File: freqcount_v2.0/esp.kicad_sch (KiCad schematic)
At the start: 1 part, among them J3 Conn_02x10_Odd_Even

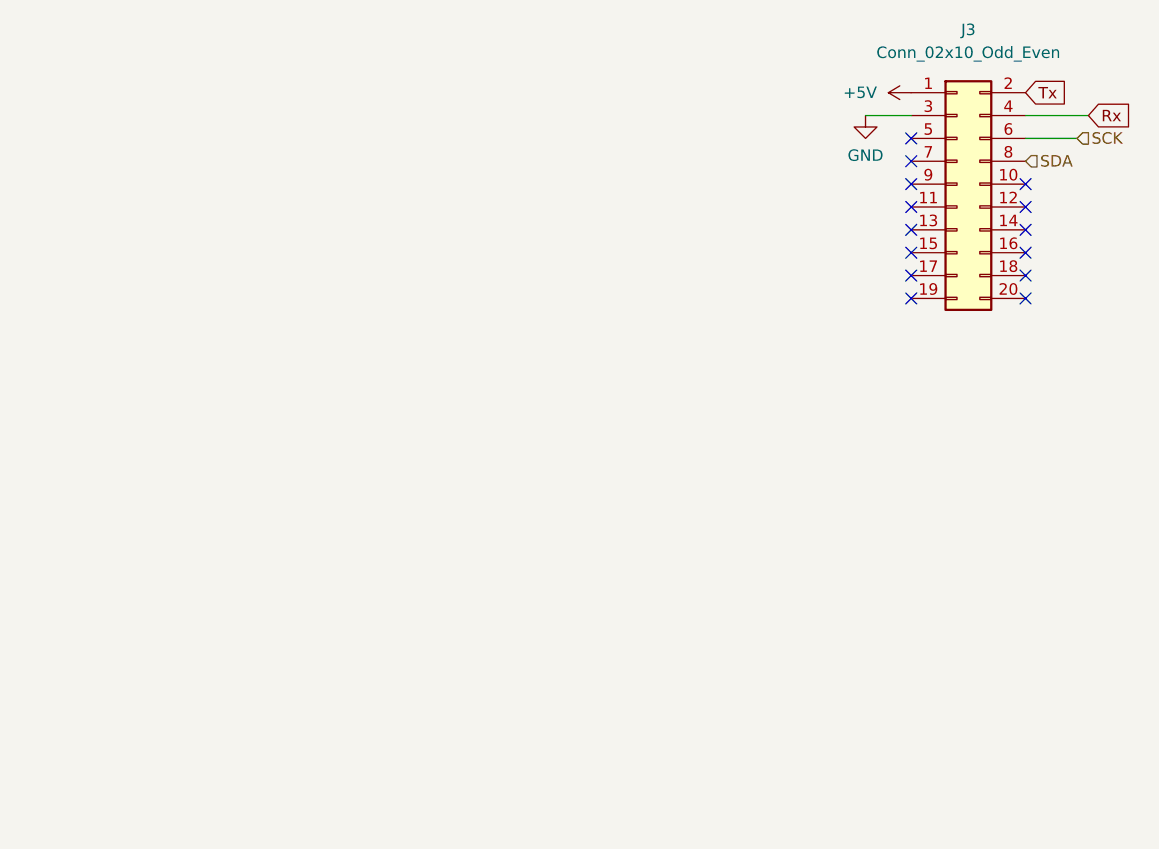
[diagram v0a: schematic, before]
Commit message: update
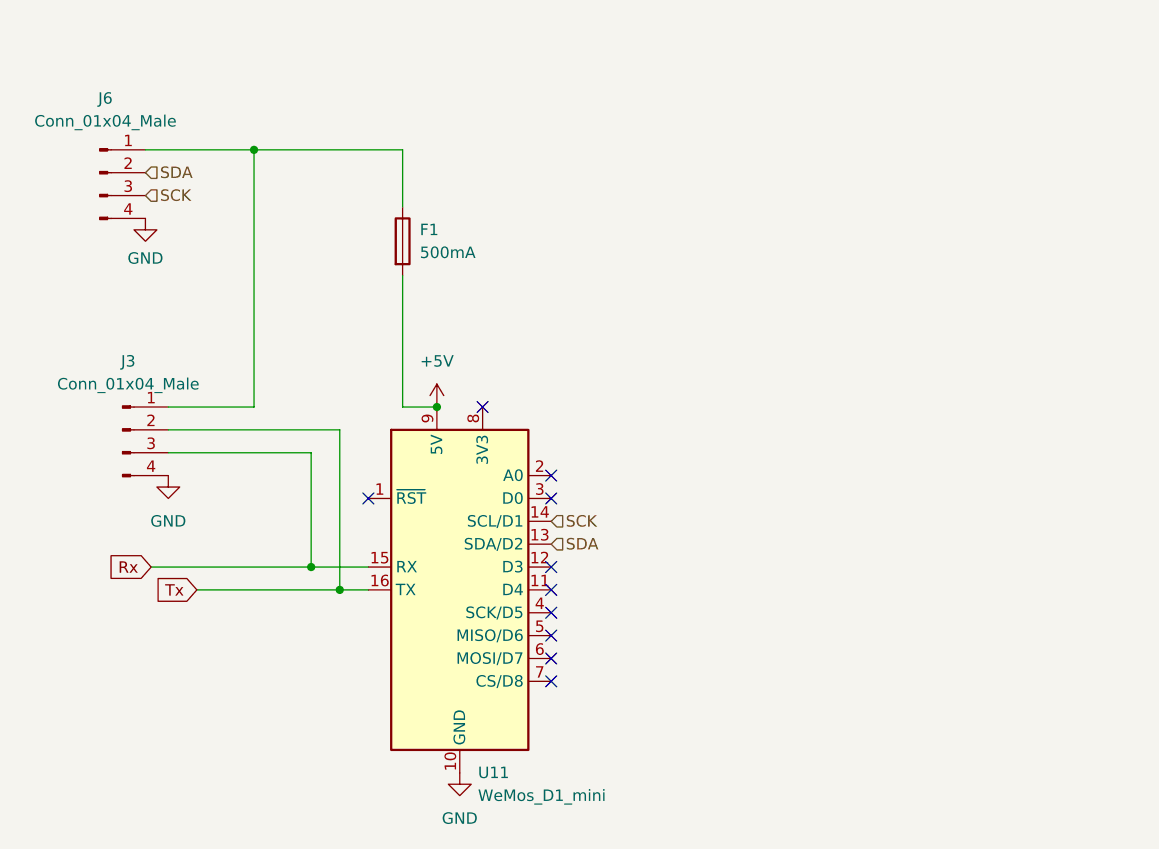
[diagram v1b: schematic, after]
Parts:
- removed J3: Conn_02x10_Odd_Even, Connector_PinHeader_2.54mm:PinHeader_2x10_P2.54mm_Vertical, symbol Connector_Generic:Conn_02x10_Odd_Even
- added F1: 500mA, Fuse:Fuseholder_TR5_Littelfuse_No560_No460, symbol Device:Fuse
- added J3, J6: Conn_01x04_Male, Connector_JST:JST_PH_B4B-PH-K_1x04_P2.00mm_Vertical, symbol Connector:Conn_01x04_Male
- added U11: WeMos_D1_mini, Module:WEMOS_D1_mini_light, symbol MCU_Module:WeMos_D1_mini
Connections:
- net +5V: now also F1.2, U11.9 (5V)
- net GND: now also J3.4 (Pin_4), J6.4 (Pin_4), U11.10 (GND)
- net Rx: now also J3.3 (Pin_3), U11.15 (RX)
- net SCK: now also J6.3 (Pin_3), U11.14 (SCL/D1)
- net SDA: now also J6.2 (Pin_2), U11.13 (SDA/D2)
- net Tx: now also J3.2 (Pin_2), U11.16 (TX)
- new net: F1.1, J3.1 (Pin_1), J6.1 (Pin_1)
- no-connect marks 14 -> 10
